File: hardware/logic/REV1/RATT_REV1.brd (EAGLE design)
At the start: 127 x 76.2 mm, 134 parts, among them IC1 MCP73832, IC10 CPC1002N, IC2 TPS2115AIPWRQ1, IC3 MAX98357, IC4 AP2112K-3.3V, IC5 PCA9539PW, IC6 TLP292-4, IC7 CPC1002N, IC8 CPC1002N, IC9 CPC1002N, J10 PHOENIX1803484, J100 RPI-ZERO, J11 PHOENIX1803484, J2 PHOENIX1803426, J3 LiPo, J4 F-1X04-SIP-100-40, J5 4P-2.0, J6 4P-2.0, J8 4P-2.0, J9 4P-2.0, Q1 2N7002

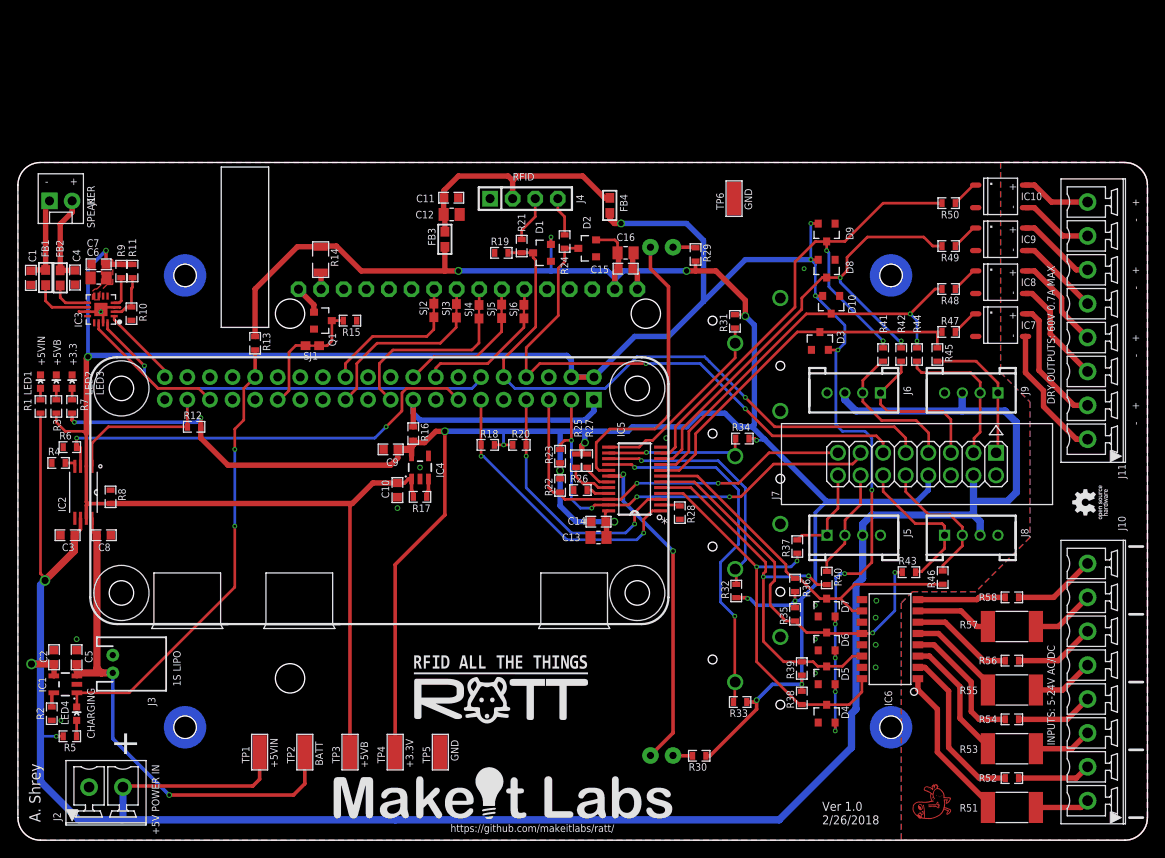
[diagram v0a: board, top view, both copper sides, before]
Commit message: Made Rev1, most changes implemented
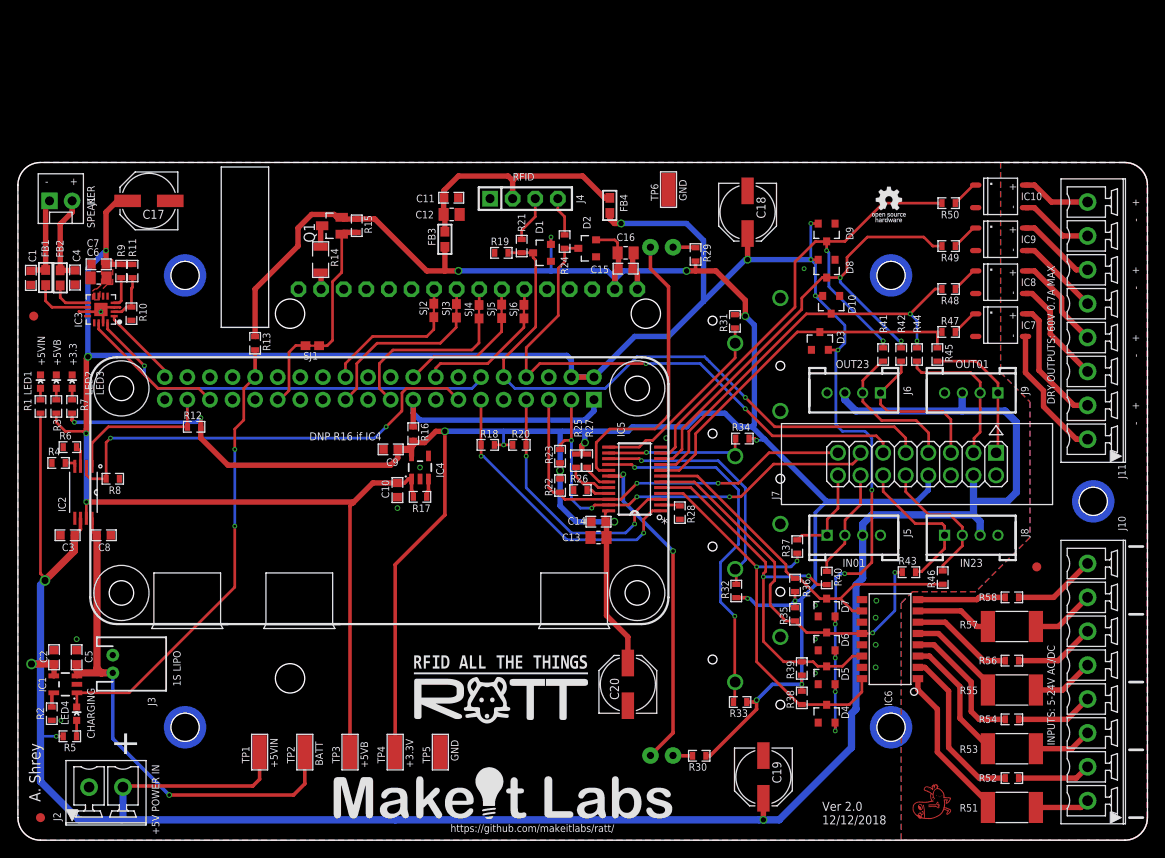
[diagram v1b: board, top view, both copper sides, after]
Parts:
- added C17, C18, C19, C20: (no value), MakeItLabs:PANASONIC_D
- added FID1, FID2, FID3: FIDUCIAL40MILX80MIL, MakeItLabs:FIDUCIAL-40MILX80MIL
- Q1: value 2N7002 -> DMP31D0U; device MakeItLabs:SOT-23 -> MakeItLabs:SOT23
- R12, R6, R8: value 10k -> 10K
- R17: value 1k -> 1K
- R19: value 1.5K -> 2K
- R2: value 2.0k -> 2K
- R21: value 750R -> 1K
- R4: value 1k -> 270R
- moved Q1 10.7 mm to (35.3, 69.1), turned to 90 degrees
- moved R15 10.7 mm to (38.1, 69.1), turned to 270 degrees
- moved TP6 7.44 mm to (73.2, 73.2)
- moved R8 2.05 mm to (10.7, 40.6), turned to 180 degrees
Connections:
- removed net N$34: LCD100.16, Q1.1
- new net N$26: IC2.3, R6.2
- new net N$3: Q1.3, R14.1
- net +3.3V: now also C20.+, Q1.2, R15.1; no longer R14.1
- net +5VB: now also C17.+, C18.+; no longer IC2.2, R8.2
- net +5VIN: now also C19.+
- net GND: now also C17.-, C18.-, C19.-, C20.-, LCD100.16; no longer Q1.2, R15.1
- net N$33: now also Q1.1; no longer Q1.3
- net SHUTDOWN: now also IC2.2, R8.2; no longer IC2.3, R6.2
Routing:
- net +3.3V: track 331.1 -> 350.3 mm
- net N$33: track 5.25 -> 15.9 mm
- net +5VB: track 291.9 -> 302.4 mm, vias 13 -> 16
- net N$34: track 3.30 -> 0.00 mm
- net N$3: track 0.00 -> 2.43 mm
- net +5VIN: track 258.8 -> 261.2 mm, vias 3 -> 4
- net N$26: track 0.00 -> 2.34 mm
- net SHUTDOWN: track 50.5 -> 51.3 mm
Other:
- board text added: "12/12/2018"
- board text added: "DNP R16 if IC4"
- board text added: "IN01"
- board text added: "IN23"
- board text added: "OUT01"
- board text added: "OUT23"
- board text added: "Ver 2.0"
- board text removed: "2/26/2018"
- board text removed: "Ver 1.0"

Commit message: REV1 as sent out to fab
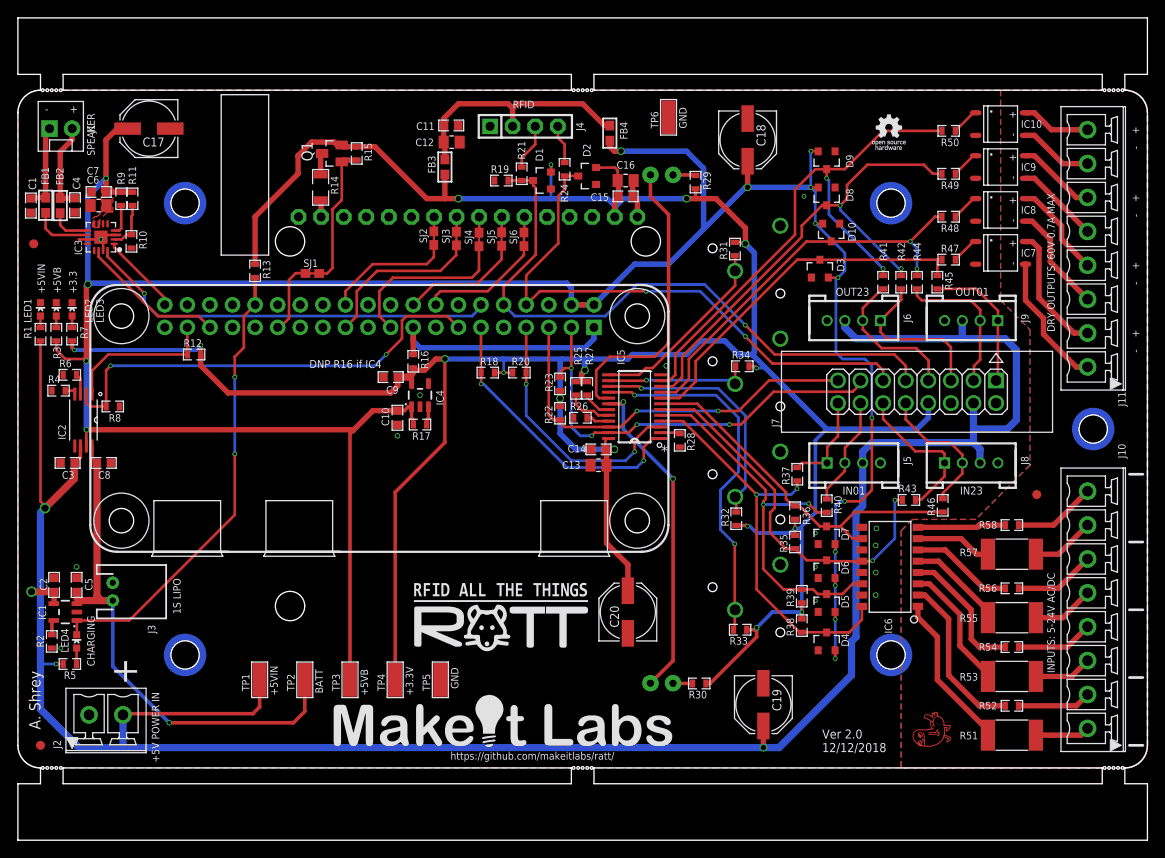
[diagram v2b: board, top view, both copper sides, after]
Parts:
- moved IC7 8.13 mm to (110.5, 66.0)
- moved R47 8.13 mm to (104.6, 65.3)
- moved SJ4 8.13 mm to (51.8, 67.5)
- moved SW103 8.13 mm to (81.9, 65.3)
- moved R46 8.13 mm to (104.0, 37.7)
- moved R5 8.13 mm to (5.84, 19.8)
- moved C10 8.13 mm to (42.7, 47.5)
- moved C11 8.13 mm to (48.7, 80.4)
- moved C12 8.13 mm to (48.8, 78.5)
- moved C13 8.13 mm to (65.3, 42.2)
- moved C14 8.13 mm to (65.3, 43.9)
- moved C15 8.13 mm to (68.3, 72.4)
- moved C16 8.13 mm to (68.3, 74.2)
- moved C17 8.13 mm to (14.7, 80.0)
- moved C18 8.13 mm to (82.0, 78.7)
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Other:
- board size 127 x 76.2 mm -> 127 x 92.5 mm
